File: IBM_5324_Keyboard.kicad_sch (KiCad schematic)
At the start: 9 parts, among them SW1 CMD, SW2 ` ~, SW3 SW_Push_45deg, SW4 SW_Push_45deg, SW5 SW_Push_45deg, SW6 SW_Push_45deg, SW7 SW_Push_45deg, SW8 SW_Push_45deg, SW9 SW_Push_45deg

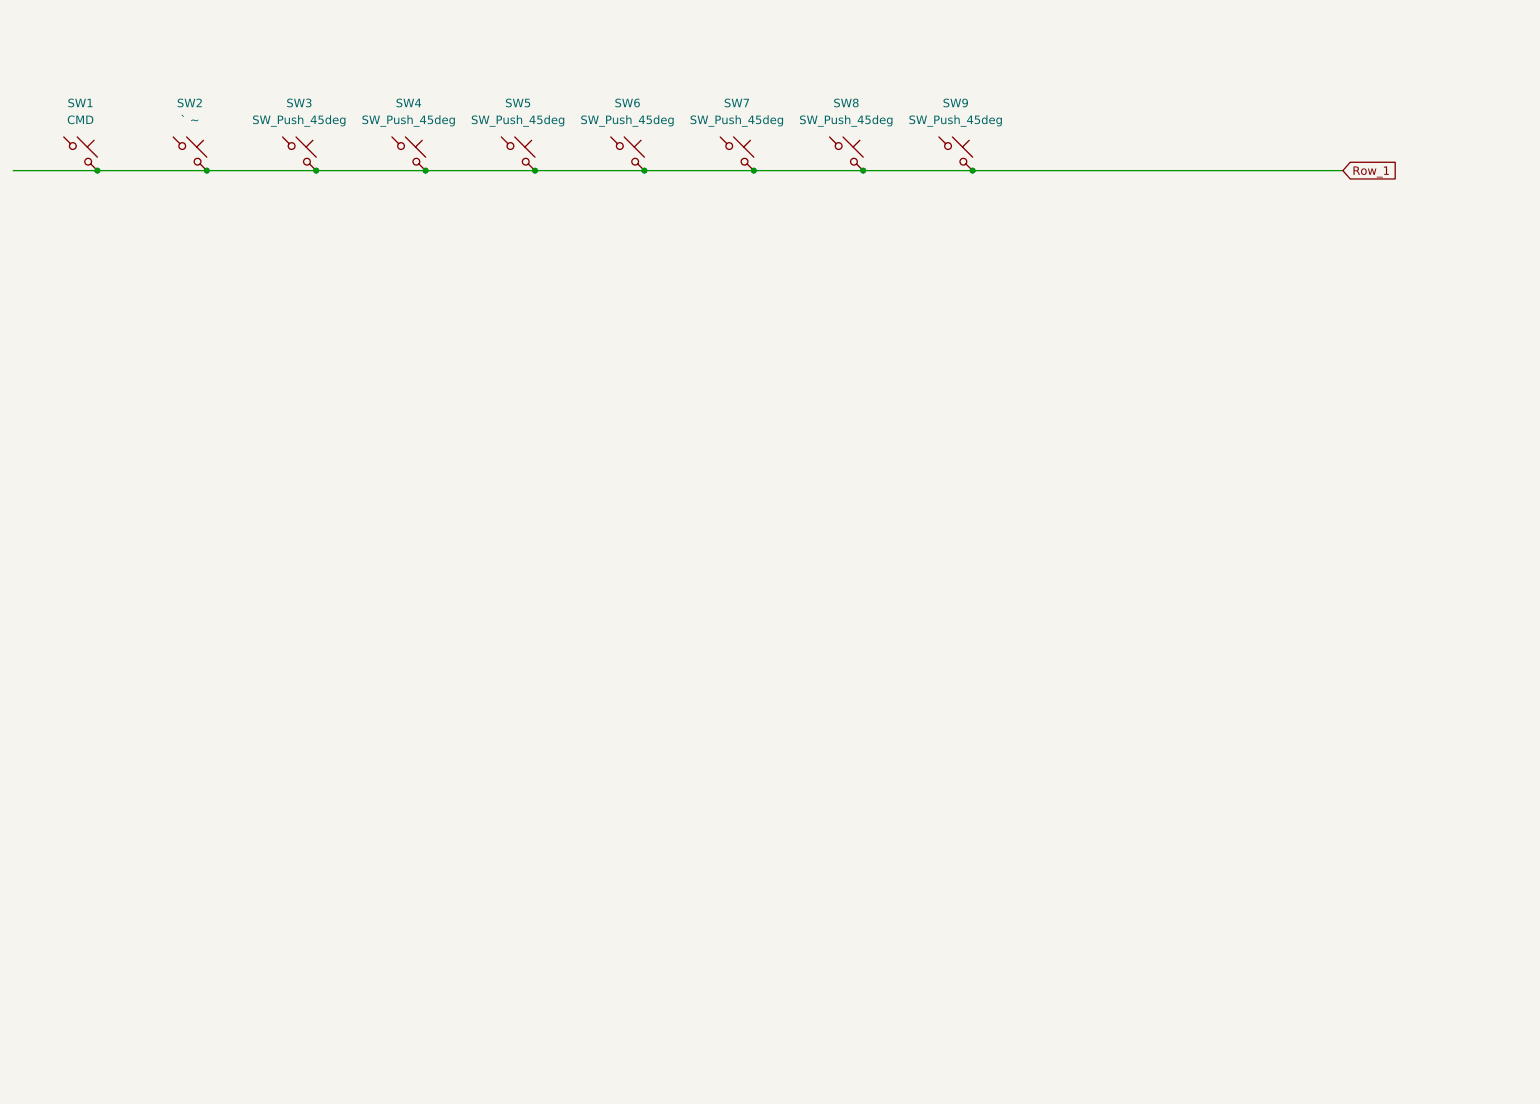
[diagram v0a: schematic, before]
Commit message: Further work
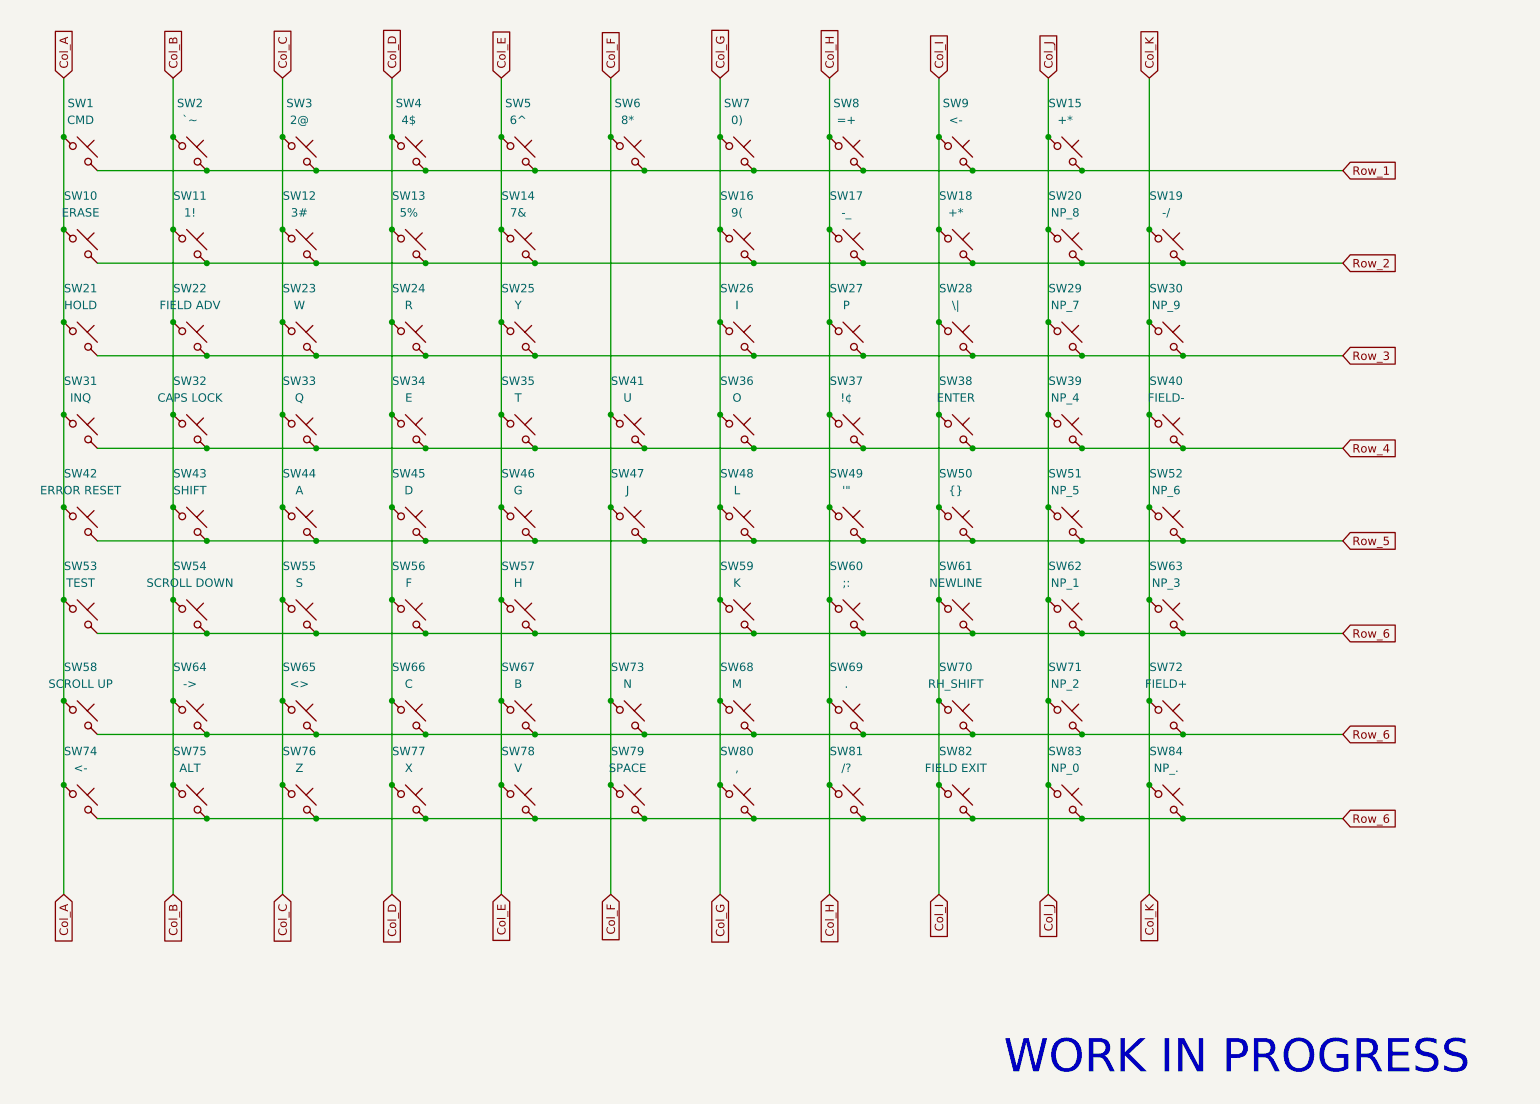
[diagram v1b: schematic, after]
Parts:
- added SW10: ERASE, symbol Switch:SW_Push_45deg
- added SW11: 1!, symbol Switch:SW_Push_45deg
- added SW12: 3#, symbol Switch:SW_Push_45deg
- added SW13: 5%, symbol Switch:SW_Push_45deg
- added SW14: 7&, symbol Switch:SW_Push_45deg
- added SW15, SW18: +*, symbol Switch:SW_Push_45deg
- added SW16: 9(, symbol Switch:SW_Push_45deg
- added SW17: -_, symbol Switch:SW_Push_45deg
- added SW19: -/, symbol Switch:SW_Push_45deg
- added SW20: NP_8, symbol Switch:SW_Push_45deg
- added SW21: HOLD, symbol Switch:SW_Push_45deg
- added SW22: FIELD ADV, symbol Switch:SW_Push_45deg
- added SW23: W, symbol Switch:SW_Push_45deg
- added SW24: R, symbol Switch:SW_Push_45deg
- added SW25: Y, symbol Switch:SW_Push_45deg
- added SW26: I, symbol Switch:SW_Push_45deg
- added SW27: P, symbol Switch:SW_Push_45deg
- added SW28: \|, symbol Switch:SW_Push_45deg
- added SW29: NP_7, symbol Switch:SW_Push_45deg
- added SW30: NP_9, symbol Switch:SW_Push_45deg
- added SW31: INQ, symbol Switch:SW_Push_45deg
- added SW32: CAPS LOCK, symbol Switch:SW_Push_45deg
- added SW33: Q, symbol Switch:SW_Push_45deg
- added SW34: E, symbol Switch:SW_Push_45deg
- added SW35: T, symbol Switch:SW_Push_45deg
- added SW36: O, symbol Switch:SW_Push_45deg
- added SW37: !¢, symbol Switch:SW_Push_45deg
- added SW38: ENTER, symbol Switch:SW_Push_45deg
- added SW39: NP_4, symbol Switch:SW_Push_45deg
- added SW40: FIELD-, symbol Switch:SW_Push_45deg
- added SW41: U, symbol Switch:SW_Push_45deg
- added SW42: ERROR RESET, symbol Switch:SW_Push_45deg
- added SW43: SHIFT, symbol Switch:SW_Push_45deg
- added SW44: A, symbol Switch:SW_Push_45deg
- added SW45: D, symbol Switch:SW_Push_45deg
- added SW46: G, symbol Switch:SW_Push_45deg
- added SW47: J, symbol Switch:SW_Push_45deg
- added SW48: L, symbol Switch:SW_Push_45deg
- added SW49: '", symbol Switch:SW_Push_45deg
- added SW50: {}, symbol Switch:SW_Push_45deg
- added SW51: NP_5, symbol Switch:SW_Push_45deg
- added SW52: NP_6, symbol Switch:SW_Push_45deg
- added SW53: TEST, symbol Switch:SW_Push_45deg
- added SW54: SCROLL DOWN, symbol Switch:SW_Push_45deg
- added SW55: S, symbol Switch:SW_Push_45deg
- added SW56: F, symbol Switch:SW_Push_45deg
- added SW57: H, symbol Switch:SW_Push_45deg
- added SW58: SCROLL UP, symbol Switch:SW_Push_45deg
- added SW59: K, symbol Switch:SW_Push_45deg
- added SW60: ;:, symbol Switch:SW_Push_45deg
- added SW61: NEWLINE, symbol Switch:SW_Push_45deg
- added SW62: NP_1, symbol Switch:SW_Push_45deg
- added SW63: NP_3, symbol Switch:SW_Push_45deg
- added SW64: ->, symbol Switch:SW_Push_45deg
- added SW65: <>, symbol Switch:SW_Push_45deg
- added SW66: C, symbol Switch:SW_Push_45deg
- added SW67: B, symbol Switch:SW_Push_45deg
- added SW68: M, symbol Switch:SW_Push_45deg
- added SW69: ., symbol Switch:SW_Push_45deg
- added SW70: RH_SHIFT, symbol Switch:SW_Push_45deg
- added SW71: NP_2, symbol Switch:SW_Push_45deg
- added SW72: FIELD+, symbol Switch:SW_Push_45deg
- added SW73: N, symbol Switch:SW_Push_45deg
- added SW74: <-, symbol Switch:SW_Push_45deg
- added SW75: ALT, symbol Switch:SW_Push_45deg
- added SW76: Z, symbol Switch:SW_Push_45deg
- added SW77: X, symbol Switch:SW_Push_45deg
- added SW78: V, symbol Switch:SW_Push_45deg
- added SW79: SPACE, symbol Switch:SW_Push_45deg
- added SW80: ,, symbol Switch:SW_Push_45deg
- added SW81: /?, symbol Switch:SW_Push_45deg
- added SW82: FIELD EXIT, symbol Switch:SW_Push_45deg
- added SW83: NP_0, symbol Switch:SW_Push_45deg
- added SW84: NP_., symbol Switch:SW_Push_45deg
- SW2: value ` ~ -> `~
- SW3: value SW_Push_45deg -> 2@
- SW4: value SW_Push_45deg -> 4$
- SW5: value SW_Push_45deg -> 6^
- SW6: value SW_Push_45deg -> 8*
- SW7: value SW_Push_45deg -> 0)
- SW8: value SW_Push_45deg -> =+
- SW9: value SW_Push_45deg -> <-
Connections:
- net Row_1: now also SW15.2
- net Col_F: now reaches SW6.1
- net Col_F: now also SW41.1, SW47.1, SW73.1, SW79.1
- net Col_B: now reaches SW2.1
- net Col_B: now also SW11.1, SW22.1, SW32.1, SW43.1, SW54.1, SW64.1, SW75.1
- net Col_C: now reaches SW3.1
- net Col_C: now also SW12.1, SW23.1, SW33.1, SW44.1, SW55.1, SW65.1, SW76.1
- net Col_I: now reaches SW9.1
- net Col_I: now also SW18.1, SW28.1, SW38.1, SW50.1, SW61.1, SW70.1, SW82.1
- net Col_A: now reaches SW1.1
- net Col_A: now also SW10.1, SW21.1, SW31.1, SW42.1, SW53.1, SW58.1, SW74.1
- net Col_H: now reaches SW8.1
- net Col_H: now also SW17.1, SW27.1, SW37.1, SW49.1, SW60.1, SW69.1, SW81.1
- net Col_D: now reaches SW4.1
- net Col_D: now also SW13.1, SW24.1, SW34.1, SW45.1, SW56.1, SW66.1, SW77.1
- net Col_E: now reaches SW5.1
- net Col_E: now also SW14.1, SW25.1, SW35.1, SW46.1, SW57.1, SW67.1, SW78.1
- net Col_G: now reaches SW7.1
- net Col_G: now also SW16.1, SW26.1, SW36.1, SW48.1, SW59.1, SW68.1, SW80.1
- new net Col_J: SW15.1, SW20.1, SW29.1, SW39.1, SW51.1, SW62.1, SW71.1, SW83.1
- new net Col_K: SW19.1, SW30.1, SW40.1, SW52.1, SW63.1, SW72.1, SW84.1
- new net Row_2: SW10.2, SW11.2, SW12.2, SW13.2, SW14.2, SW16.2, SW17.2, SW18.2, SW19.2, SW20.2
- new net Row_3: SW21.2, SW22.2, SW23.2, SW24.2, SW25.2, SW26.2, SW27.2, SW28.2, SW29.2, SW30.2
- new net Row_4: SW31.2, SW32.2, SW33.2, SW34.2, SW35.2, SW36.2, SW37.2, SW38.2, SW39.2, SW40.2, SW41.2
- new net Row_5: SW42.2, SW43.2, SW44.2, SW45.2, SW46.2, SW47.2, SW48.2, SW49.2, SW50.2, SW51.2, SW52.2
- new net Row_6: SW53.2, SW54.2, SW55.2, SW56.2, SW57.2, SW58.2, SW59.2, SW60.2, SW61.2, SW62.2, SW63.2, SW64.2, SW65.2, SW66.2, SW67.2, SW68.2, SW69.2, SW70.2, SW71.2, SW72.2, SW73.2, SW74.2, SW75.2, SW76.2, SW77.2, SW78.2, SW79.2, SW80.2, SW81.2, SW82.2, SW83.2, SW84.2
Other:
- note added: "WORK IN PROGRESS"
